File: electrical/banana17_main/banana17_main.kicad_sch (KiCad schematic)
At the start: 29 parts, among them J1 USB_C_Receptacle_USB2.0_16P, U1 RP2040, U2 NCP1117-3.3_SOT223, U3 ssd1306_128x32, U4 W25Q128JVS, Y1 ABMB-272-T3

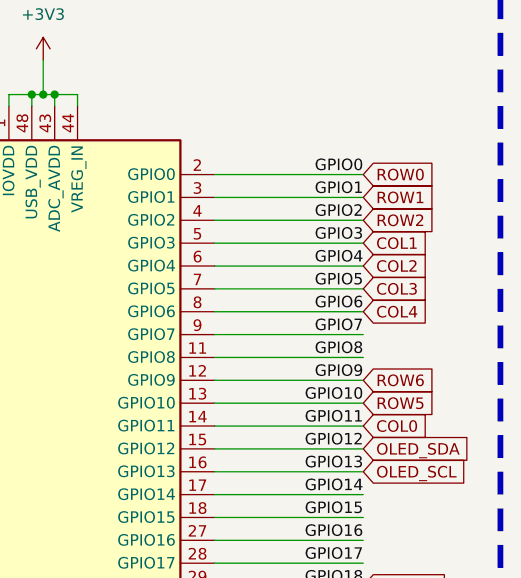
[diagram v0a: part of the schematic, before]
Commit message: Additional changes to routing.
Additional changes to routing.
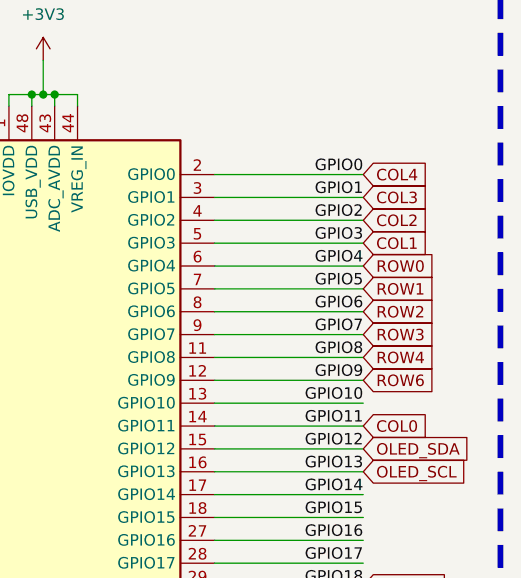
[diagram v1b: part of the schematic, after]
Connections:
- net COL2: now also U1.4 (GPIO2); no longer U1.6 (GPIO4)
- net COL3: now also U1.3 (GPIO1); no longer U1.7 (GPIO5)
- net COL4: now also U1.2 (GPIO0); no longer U1.8 (GPIO6)
- net ROW0: now also U1.6 (GPIO4); no longer U1.2 (GPIO0)
- net ROW1: now also U1.7 (GPIO5); no longer U1.3 (GPIO1)
- net ROW2: now also U1.8 (GPIO6); no longer U1.4 (GPIO2)
- net GPIO7 renamed ROW3
- net GPIO8 renamed ROW4
- net ROW5 renamed GPIO10

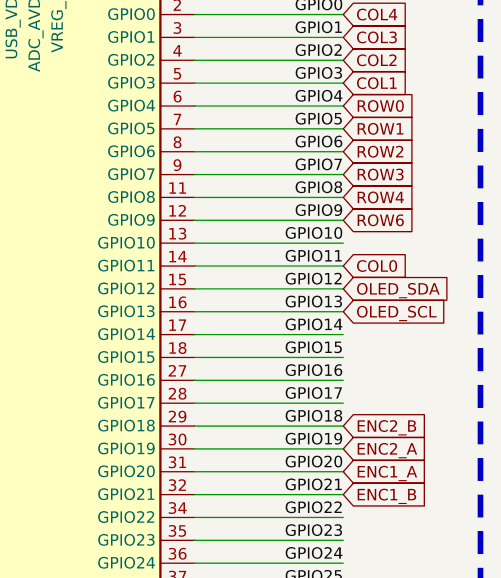
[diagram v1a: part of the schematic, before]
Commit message: Tracks rerouted.
Tracks rerouted.
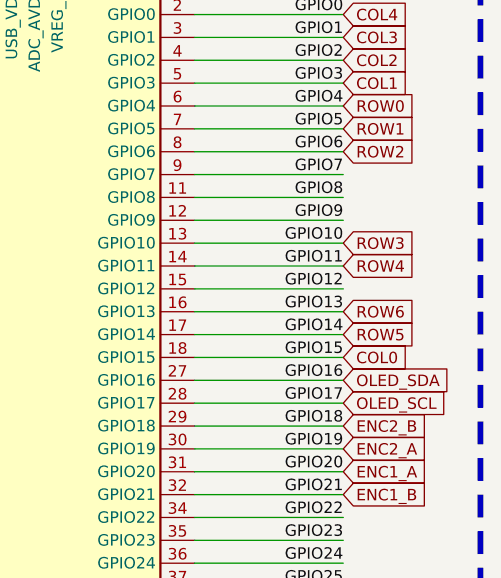
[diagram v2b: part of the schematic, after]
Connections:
- net GPIO10 is gone; now on net ROW3: U1.13 (GPIO10)
- net GPIO15 is gone; now on net COL0: U1.18 (GPIO15)
- net GPIO16 is gone; now on net OLED_SDA: U1.27 (GPIO16)
- net GPIO17 is gone; now on net OLED_SCL: U1.28 (GPIO17)
- net COL0: no longer U1.14 (GPIO11)
- net OLED_SCL: no longer U1.16 (GPIO13)
- net OLED_SDA: no longer U1.15 (GPIO12)
- net ROW3: no longer U1.9 (GPIO7)
- net ROW4: now also U1.14 (GPIO11); no longer U1.11 (GPIO8)
- net ROW6: now also U1.16 (GPIO13); no longer U1.12 (GPIO9)
- net GPIO14 renamed ROW5
- new net GPIO12: U1.15 (GPIO12)
- new net GPIO7: U1.9 (GPIO7)
- new net GPIO8: U1.11 (GPIO8)
- new net GPIO9: U1.12 (GPIO9)
